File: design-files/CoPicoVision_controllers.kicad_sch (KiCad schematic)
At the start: 2 parts, among them J401 DE9_Plug_MountingHoles, J402 DE9_Plug_MountingHoles

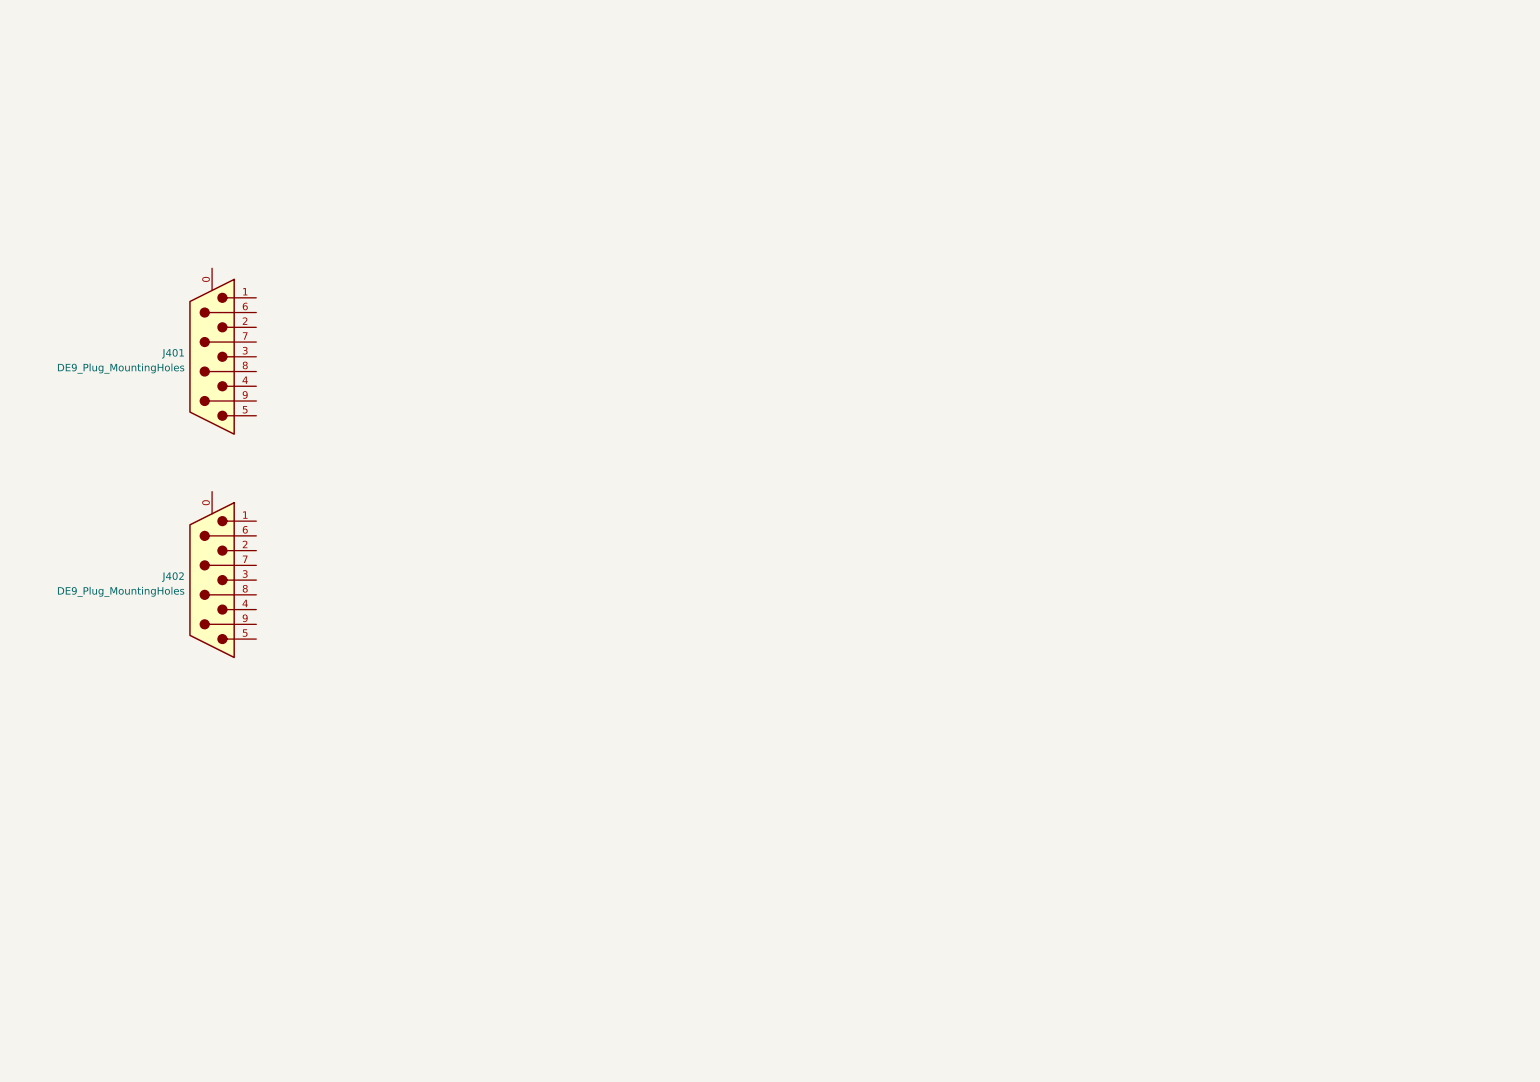
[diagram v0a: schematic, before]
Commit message: Checkpoint on controller circuit.
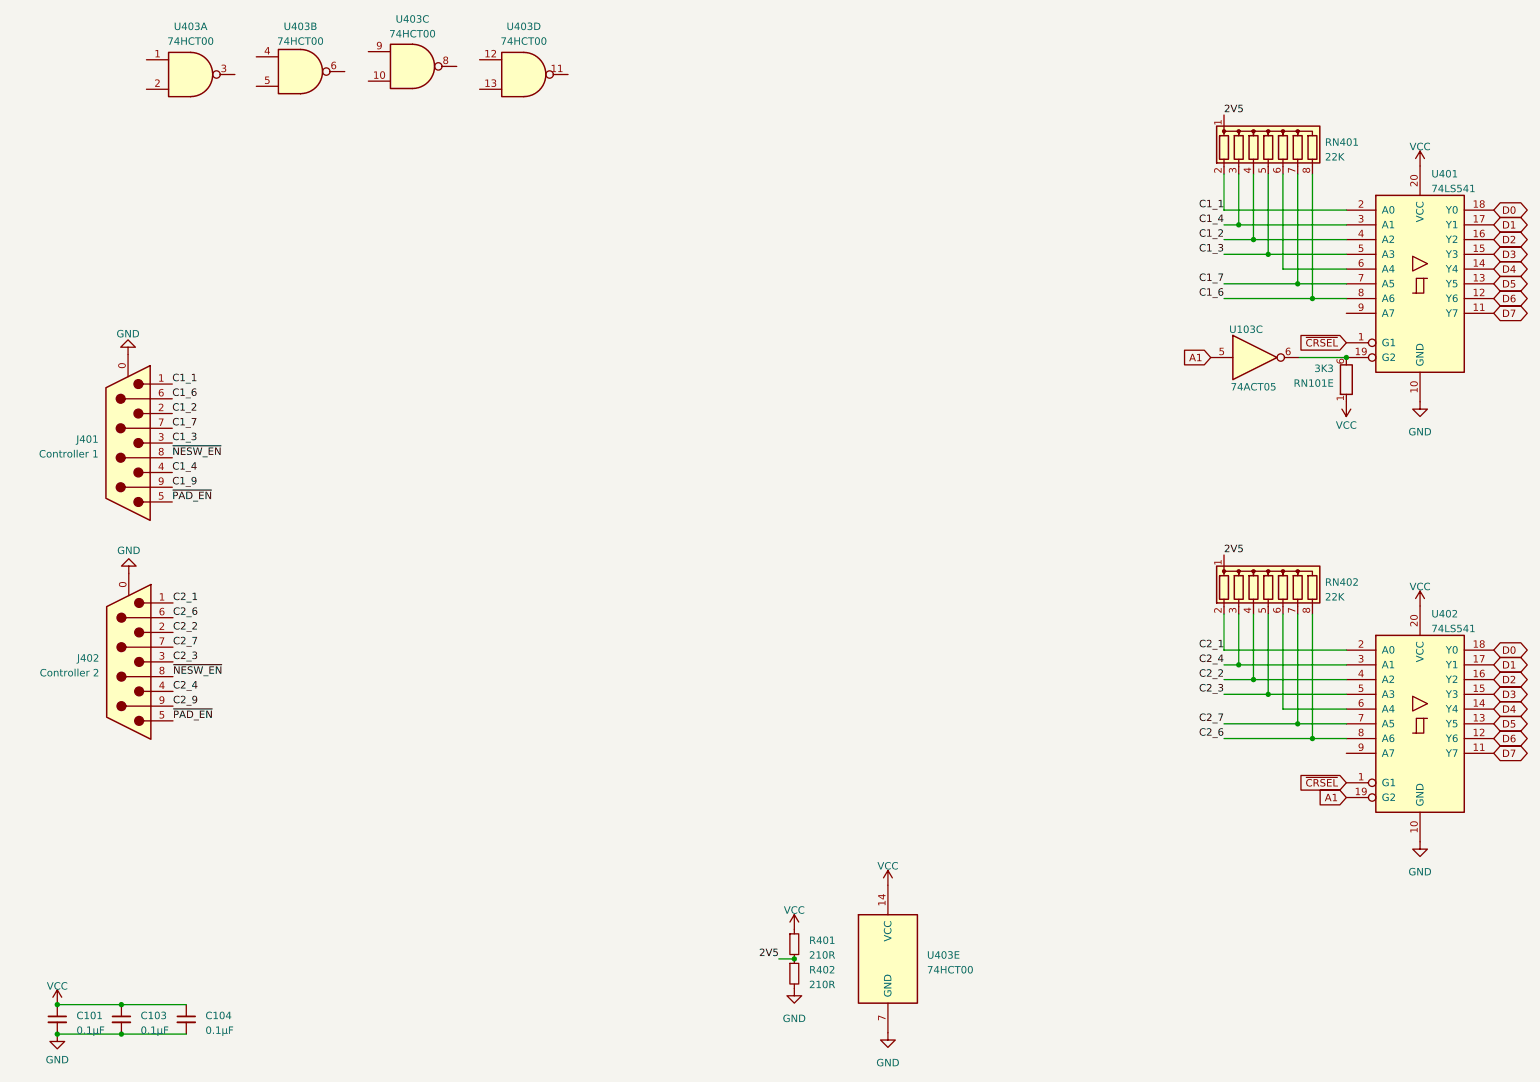
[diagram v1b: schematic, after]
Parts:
- added C101, C103, C104: 0.1µF, Capacitor_THT:C_Disc_D3.8mm_W2.6mm_P2.50mm, symbol Device:C_Small
- added R401, R402: 210R, Resistor_THT:R_Axial_DIN0207_L6.3mm_D2.5mm_P7.62mm_Horizontal, symbol Device:R_Small
- added RN101: 3K3, Resistor_THT:R_Array_SIP9, symbol Device:R_Network08_Split
- added RN401, RN402: 22K, Resistor_THT:R_Array_SIP8, symbol Device:R_Network07
- added U103: 74ACT05, Package_DIP:DIP-14_W7.62mm_Socket, symbol 74xx:74LS05
- added U401, U402: 74LS541, Package_DIP:DIP-20_W7.62mm_Socket, symbol 74xx:74LS541
- added U403: 74HCT00, Package_DIP:DIP-14_W7.62mm_Socket, symbol 74xx:74HCT00
- J401: value DE9_Plug_MountingHoles -> Controller 1
- J402: value DE9_Plug_MountingHoles -> Controller 2
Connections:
- net GND: now reaches J401.0 (PAD)
- net GND: now also J402.0 (PAD), C101.2, C103.2, C104.2, R402.2, U401.10 (GND), U402.10 (GND), U403.7 (GND)
- net C1_1: now reaches J401.1
- net C1_1: now also RN401.2 (R1), U401.2 (A0)
- net C1_2: now reaches J401.2
- net C1_2: now also RN401.4 (R3), U401.4 (A2)
- net C1_3: now reaches J401.3
- net C1_3: now also RN401.5 (R4), U401.5 (A3)
- net C1_4: now reaches J401.4
- net C1_4: now also RN401.3 (R2), U401.3 (A1)
- net ~{PAD_EN}: now reaches J401.5
- net ~{PAD_EN}: now also J402.5
- net C1_6: now reaches J401.6
- net C1_6: now also RN401.8 (R7), U401.8 (A6)
- net C1_7: now reaches J401.7
- net C1_7: now also RN401.7 (R6), U401.7 (A5)
- net ~{NESW_EN}: now reaches J401.8
- net ~{NESW_EN}: now also J402.8
- net C1_9: now reaches J401.9
- net C2_1: now reaches J402.1
- net C2_1: now also RN402.2 (R1), U402.2 (A0)
- net C2_2: now reaches J402.2
- net C2_2: now also RN402.4 (R3), U402.4 (A2)
- net C2_3: now reaches J402.3
- net C2_3: now also RN402.5 (R4), U402.5 (A3)
- net C2_4: now reaches J402.4
- net C2_4: now also RN402.3 (R2), U402.3 (A1)
- net C2_6: now reaches J402.6
- net C2_6: now also RN402.8 (R7), U402.8 (A6)
- net C2_7: now reaches J402.7
- net C2_7: now also RN402.7 (R6), U402.7 (A5)
- net C2_9: now reaches J402.9
- new net: RN402.6 (R5), U402.6 (A4)
- new net: RN401.6 (R5), U401.6 (A4)
- new net: RN101.6 (R5.2), U103.6, U401.19 (G2)
- new net 2V5: R401.2, R402.1, RN401.1 (common), RN402.1 (common)
- new net A1: U103.5, U402.19 (G2)
- new net D0: U401.18 (Y0), U402.18 (Y0)
- new net D1: U401.17 (Y1), U402.17 (Y1)
- new net D2: U401.16 (Y2), U402.16 (Y2)
- new net D3: U401.15 (Y3), U402.15 (Y3)
- new net D4: U401.14 (Y4), U402.14 (Y4)
- new net D5: U401.13 (Y5), U402.13 (Y5)
- new net D6: U401.12 (Y6), U402.12 (Y6)
- new net D7: U401.11 (Y7), U402.11 (Y7)
- new net VCC: C101.1, C103.1, C104.1, R401.1, RN101.1 (R1), U401.20 (VCC), U402.20 (VCC), U403.14 (VCC)
- new net ~{CRSEL}: U401.1 (G1), U402.1 (G1)
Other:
- moved on the sheet: J401, J402

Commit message: Controller circuit checkpoint.
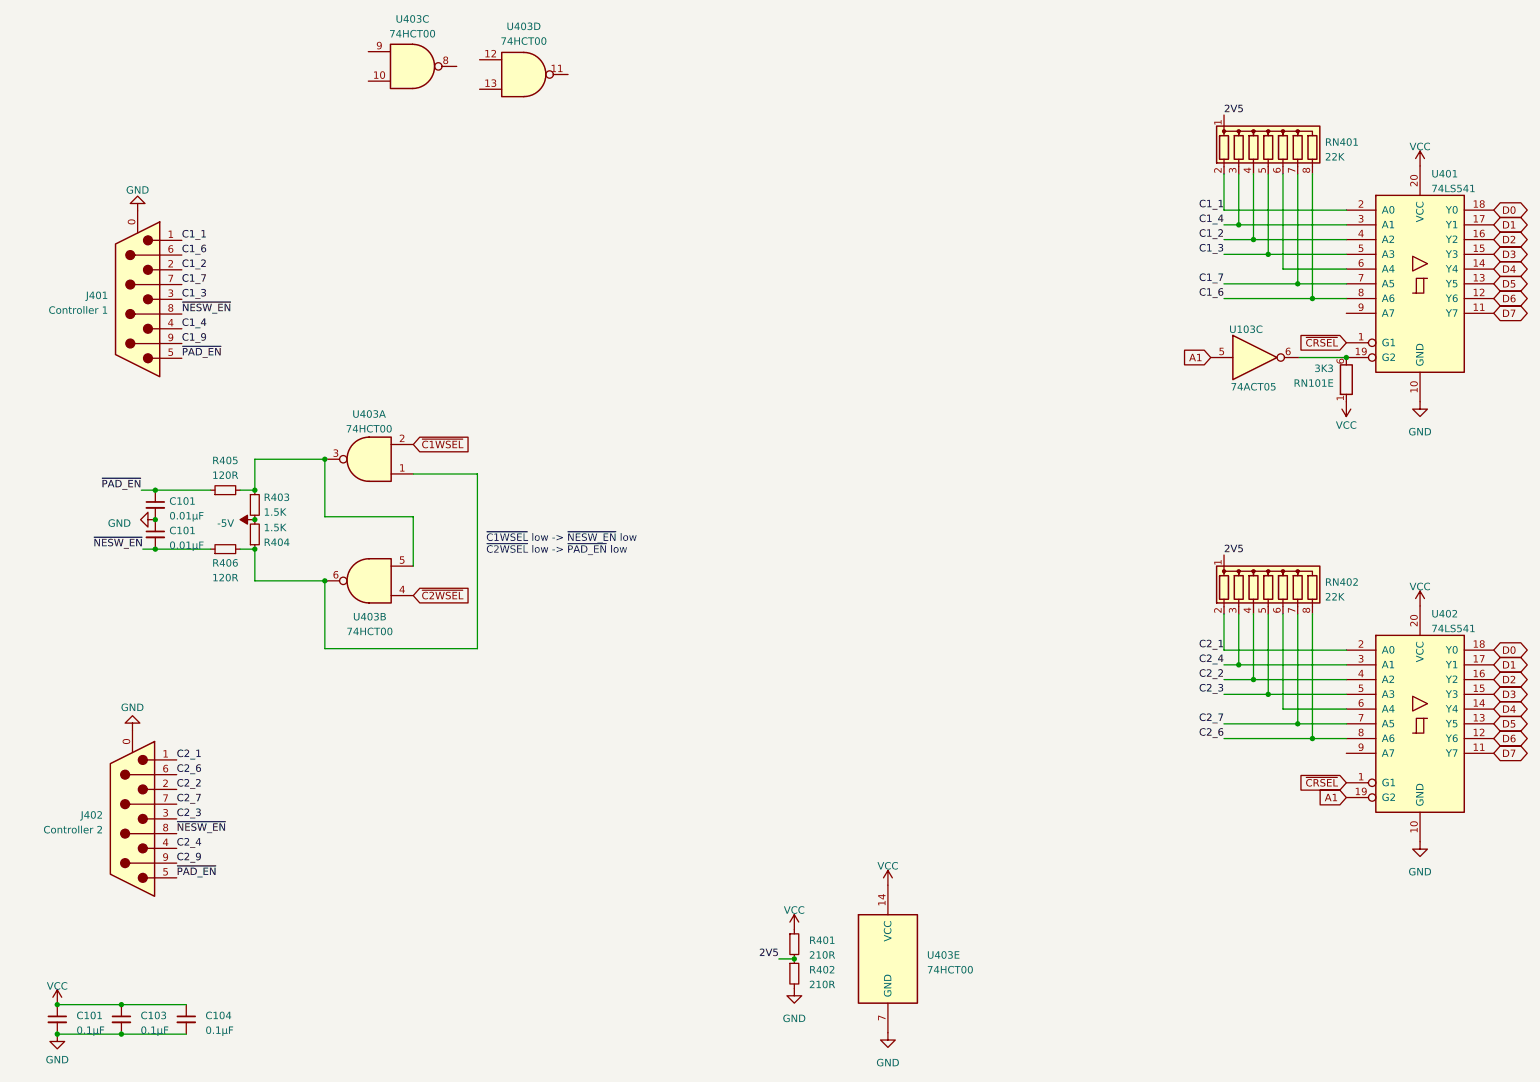
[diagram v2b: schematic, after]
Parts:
- added C101 (x2): 0.01µF, Capacitor_THT:C_Disc_D3.8mm_W2.6mm_P2.50mm, symbol Device:C_Small
- added R403, R404: 1.5K, Resistor_THT:R_Axial_DIN0207_L6.3mm_D2.5mm_P7.62mm_Horizontal, symbol Device:R_Small
- added R405, R406: 120R, Resistor_THT:R_Axial_DIN0207_L6.3mm_D2.5mm_P7.62mm_Horizontal, symbol Device:R_Small
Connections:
- net GND: now also C101.1, C101.2
- net ~{NESW_EN}: now also C101.2, R406.1
- net ~{PAD_EN}: now also C101.1, R405.1
- net at U403.1: now also U403.6, R404.1, R406.2
- net ~{C1WSEL}: now reaches U403.2
- net at U403.3: now also U403.5, R403.1, R405.2
- net ~{C2WSEL}: now reaches U403.4
- new net -5V: R403.2, R404.2
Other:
- note added: "~{C1WSEL} low -> ~{NESW_EN} low ~{C2WSEL} low -> ~{PAD_EN} low"
- moved on the sheet: J401, J402, U403A, U403B
